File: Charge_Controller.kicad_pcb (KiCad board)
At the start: 2 copper layers, 134.6 x 76.2 mm, 156 parts, among them J1 SOLAR, J10 Conn_01x01_Female, J11 Conn_01x01_Female, J12 Conn_01x01_Female, J13 Conn_01x01_Female, J14 Conn_01x01_Female, J15 Conn_01x01_Female, J16 Conn_01x01_Female, J17 Conn_01x01_Female, J18 Conn_01x01_Female, J19 Conn_01x01_Female, J2 Conn_01x01_Female, J20 Conn_01x01_Female, J21 Conn_01x01_Female, J22 Conn_01x01_Female, J23 Conn_01x01_Female, J24 Conn_01x01_Female, J25 Conn_01x01_Female, J26 Conn_01x01_Female, J27 Conn_01x01_Female, J28 Conn_01x01_Female, J29 Conn_01x01_Female, J3 Conn_01x01_Female, J30 Conn_01x01_Female, J31 Conn_01x01_Female, J32 Conn_01x01_Female, J33 Conn_01x01_Female, J34 Conn_01x01_Female, J36 FAN, J38 I2C_CON, J4 Conn_01x01_Female, J5 Conn_01x01_Female, J6 Conn_01x01_Female, J7 Conn_01x01_Female, J8 BATT, J9 USB_OTG, Q1 CSD19505, Q2 CSD19505, Q3 CSD19505, Q4 Si2306, Q5 2N3904, Q6 2N3904, Q7 PMOS-100V-78A, Q8 PMOS-100V-78A, Q9 Si2306, SW1 RIGHT, SW2 LEFT, SW3 BACK, SW4 SELECT, U1 ACS712-30A, U10 ADS1015, U11 NUP4202, U12 PCF8574, U2 B1212, U3 AMS1117-5.0, U4 AMS1117-3.3, U5 XL7005A, U6 XL7005A, U7 IR2104, U8 ESP32-WROOM-32, U9 CH340C

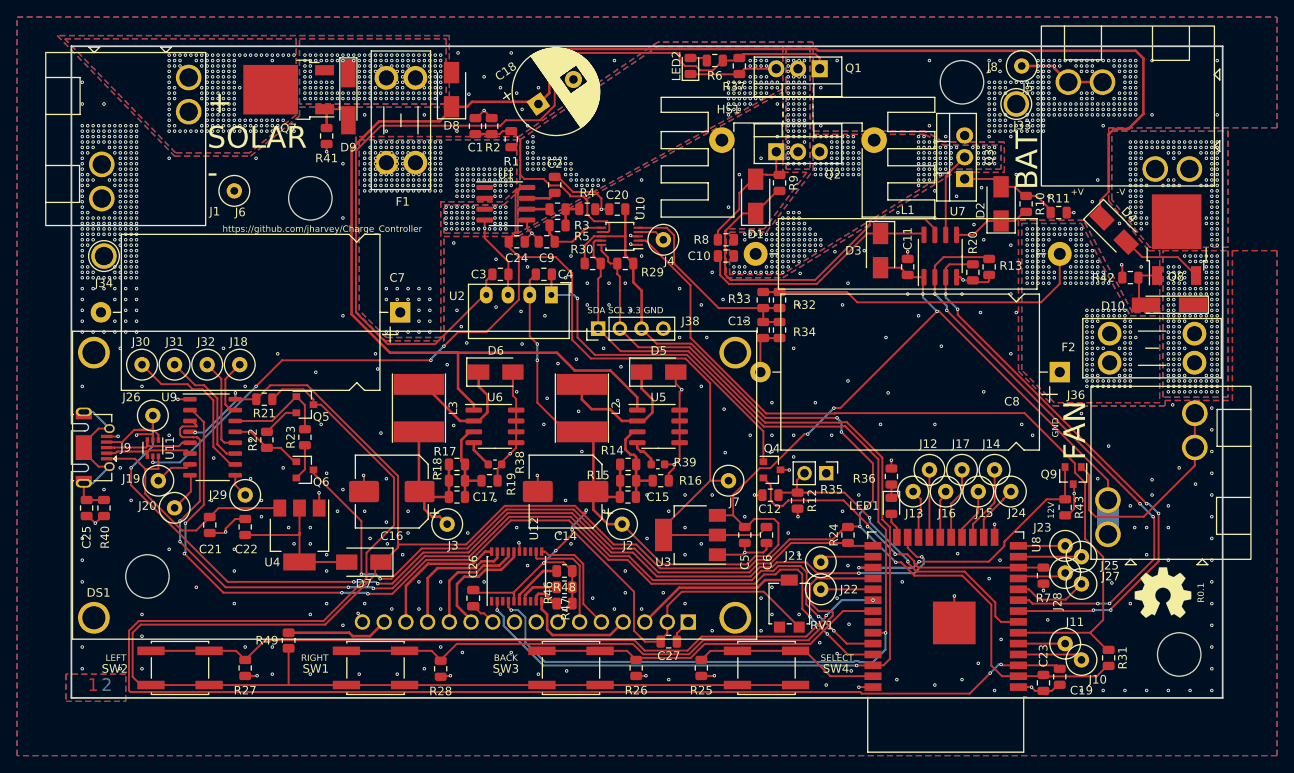
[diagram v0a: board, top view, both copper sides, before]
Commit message: Potentially going to release this as the first spin.
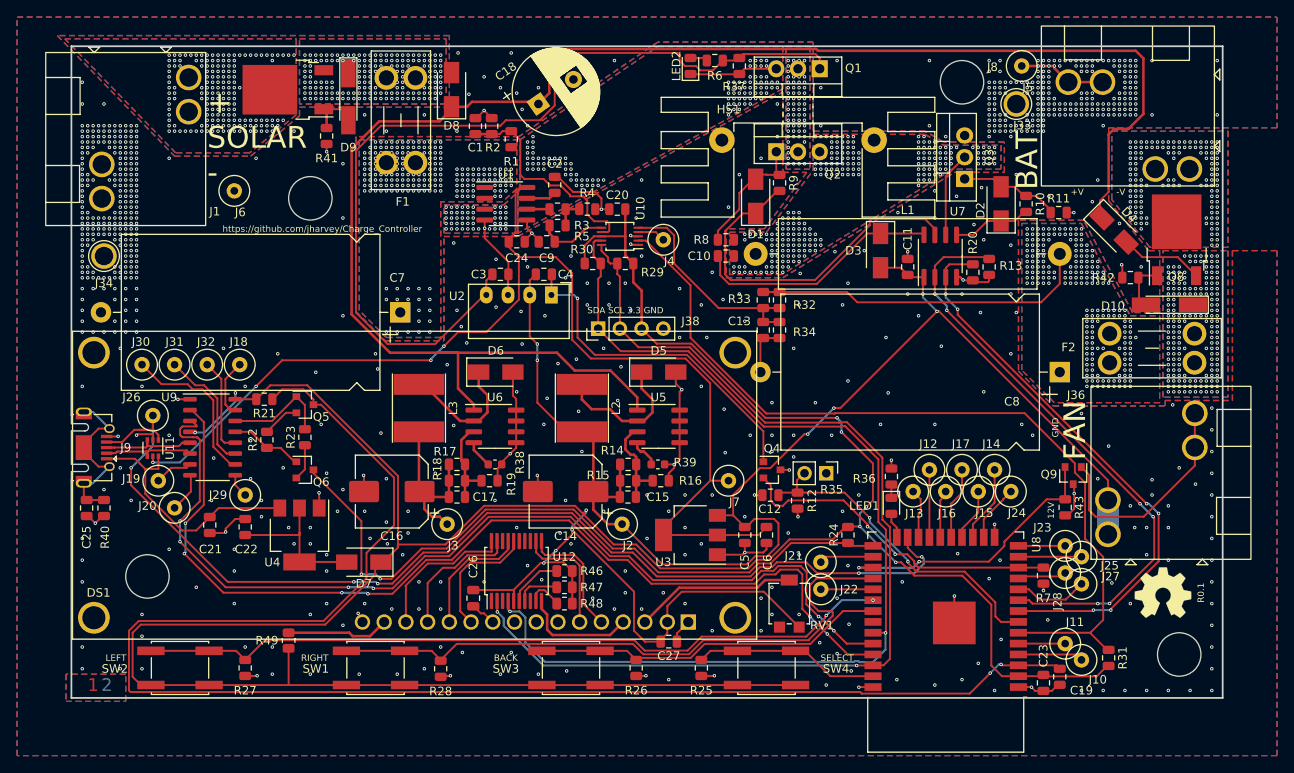
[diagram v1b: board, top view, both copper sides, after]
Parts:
- U12: footprint Package_SO:SSOP-20_4.4x6.5mm_P0.65mm -> Package_SO:SSOP-20_5.3x7.2mm_P0.65mm
- moved Q2 2.54 mm to (151.4, 80.2)
- moved Q3 2.54 mm to (170.9, 80.8)
- moved Q1 2.54 mm to (151.4, 70.5)
- moved Q8 1.12 mm to (195.7, 91.6)
- moved Q7 1.02 mm to (92.9, 72.9)
- moved U12 0.64 mm to (118.5, 129.2), turned to 0 degrees
- turned RV1 to 0 degrees
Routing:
- net Net-(DS1-Pad14): track 15.9 -> 17.2 mm
- net /RW: track 13.1 -> 14.4 mm
- net GND: track 131.9 -> 130.9 mm, vias 789 -> 788
- net +3.3VA: track 399.4 -> 398.5 mm
- net Net-(DS1-Pad11): track 13.7 -> 14.6 mm
- net Net-(DS1-Pad12): track 13.5 -> 14.4 mm
- net /E: track 12.8 -> 13.7 mm
- net Net-(R48-Pad2): track 3.59 -> 4.20 mm
- net Net-(DS1-Pad13): track 15.0 -> 15.5 mm
